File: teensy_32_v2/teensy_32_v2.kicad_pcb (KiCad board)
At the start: 2 copper layers, 65 x 56.5 mm, 62 parts, among them J1 277-1667-ND, J2 277-1667-ND, J3 CJ, J4 CJ, J5 CJ, J6 CJ, J7 M20-9980845, J8 M20-9970445, J9 TSW-108-07-G-T, P1 S9200-ND, Q1 STL60P4LLF6, U1 TEENSY, U2 MF-DSC-SOT233-BSS138, U3 RT7257G, U4 PCF8563TS/5,118, Y1 SC20S-12.5PF20PPM

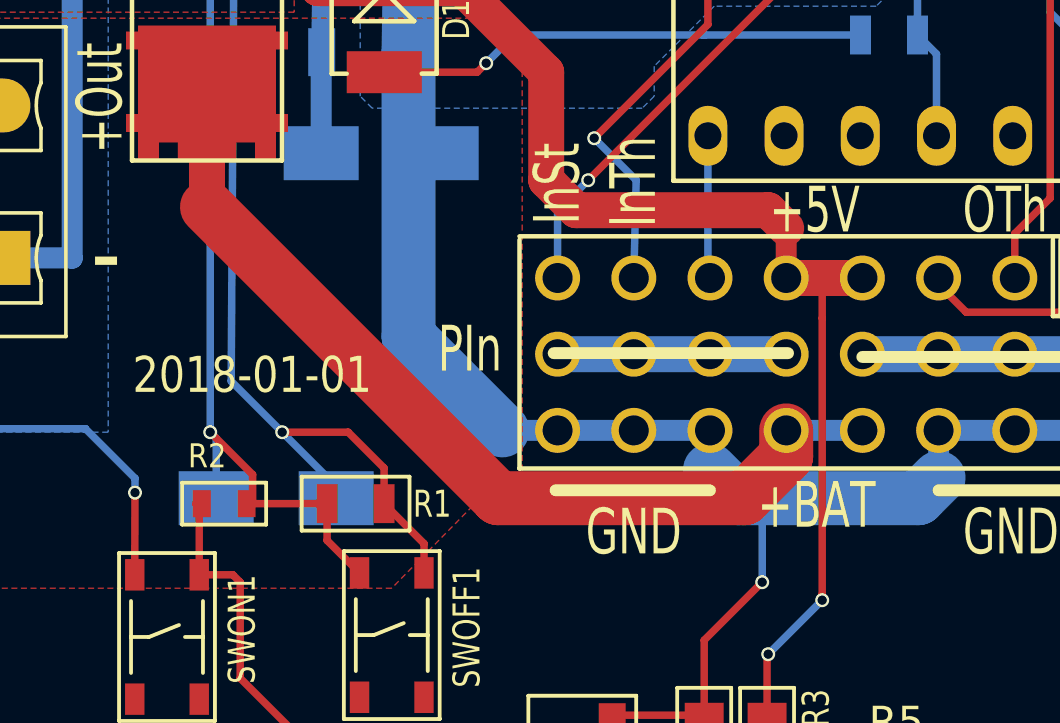
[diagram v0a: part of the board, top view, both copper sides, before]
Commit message: more work on teensy shield
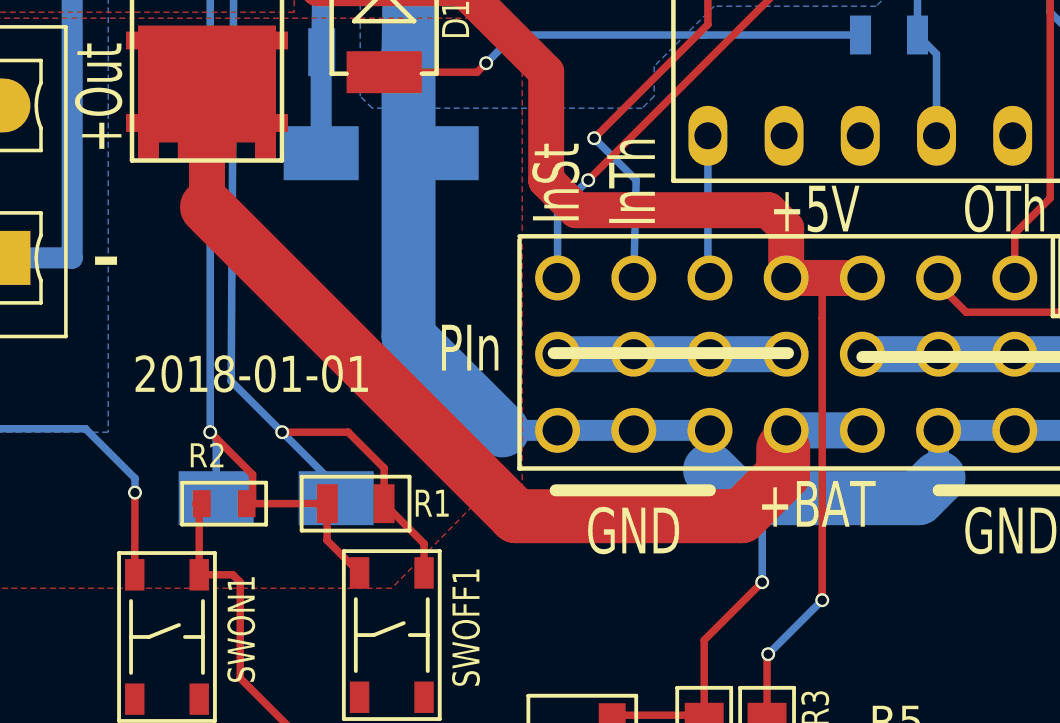
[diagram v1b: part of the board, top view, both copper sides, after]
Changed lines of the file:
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@@
     (links 166)
     (no_connects 0)
-    (area 74.949999 59.949999 140.050001 116.550001)
+    (area 69.523819 58.652 146.962016 123.037092)
     (thickness 1.6)
     (drawings 87)
@@
   (page A4)
   (layers
-    (0 F.Cu signal hide)
+    (0 F.Cu signal)
     (31 B.Cu signal)
     (32 B.Adhes user hide)
@@
   )
   (setup
-    (last_trace_width 0.7)
+    (last_trace_width 1.2)
     (user_trace_width 0.25)
     (user_trace_width 0.45)
@@
     (pad_to_mask_clearance 0)
     (aux_axis_origin 0 0)
-    (visible_elements 7FFEBF7F)
+    (visible_elements 7FFEFF7F)
     (pcbplotparams
       (layerselection 0x010fc_80000001)
@@
   (segment (start 87.884 77.681) (end 86.319 77.681) (width 1.2) (layer F.Cu) (net 2))
   (segment (start 86.319 77.681) (end 84.2 79.8) (width 1.2) (layer F.Cu) (net 2))
-  (segment (start 107 96.8) (end 107 98.46) (width 0.7) (layer F.Cu) (net 2))
+  (segment (start 107 96.8) (end 107 98.46) (width 1.2) (layer F.Cu) (net 2))
   (segment (start 106.4 96.2) (end 107 96.8) (width 1.2) (layer F.Cu) (net 2))
   (segment (start 100 96.2) (end 106.4 96.2) (width 1.2) (layer F.Cu) (net 2))
@@
   (via (at 97 91.3) (size 0.465) (drill 0.31) (layers F.Cu B.Cu) (net 81))
   (segment (start 97.9395 90.3605) (end 97 91.3) (width 0.25) (layer B.Cu) (net 81))
-  (segment (start 107 103.54) (end 107 104.4) (width 1.8) (layer F.Cu) (net 81))
+  (segment (start 106.9 104.14) (end 106.9 105) (width 1.8) (layer F.Cu) (net 81))
   (segment (start 87.6935 96.0935) (end 87.6935 91.993) (width 1.2) (layer F.Cu) (net 81))
-  (segment (start 97.4 105.8) (end 87.6935 96.0935) (width 1.8) (layer F.Cu) (net 81))
-  (segment (start 105.6 105.8) (end 97.4 105.8) (width 1.8) (layer F.Cu) (net 81))
-  (segment (start 107 104.4) (end 105.6 105.8) (width 1.8) (layer F.Cu) (net 81))
-  (segment (start 107 103.54) (end 109.54 103.54) (width 0.7) (layer B.Cu) (net 81))
+  (segment (start 98 106.4) (end 87.6935 96.0935) (width 1.8) (layer F.Cu) (net 81))
+  (segment (start 105.5 106.4) (end 98 106.4) (width 1.8) (layer F.Cu) (net 81))
+  (segment (start 106.9 105) (end 105.5 106.4) (width 1.8) (layer F.Cu) (net 81))
+  (segment (start 107 103.54) (end 109.54 103.54) (width 1.2) (layer B.Cu) (net 81))
   (segment (start 109.47654 90.3605) (end 104.3 90.3605) (width 0.25) (layer B.Cu) (net 81))
   (segment (start 104.3 90.3605) (end 104.2395 90.3605) (width 0.25) (layer B.Cu) (net 81))
